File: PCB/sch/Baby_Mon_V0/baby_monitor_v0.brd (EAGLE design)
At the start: 20 x 20 mm, 40 parts, among them J1 BATT-COIN1CR1216, U1 NRF5340-QKAA-AB0-R, U2 MAX30101EFD+, U3 MAX30205MTA+, X1 XRCGB32M000F2P10R0

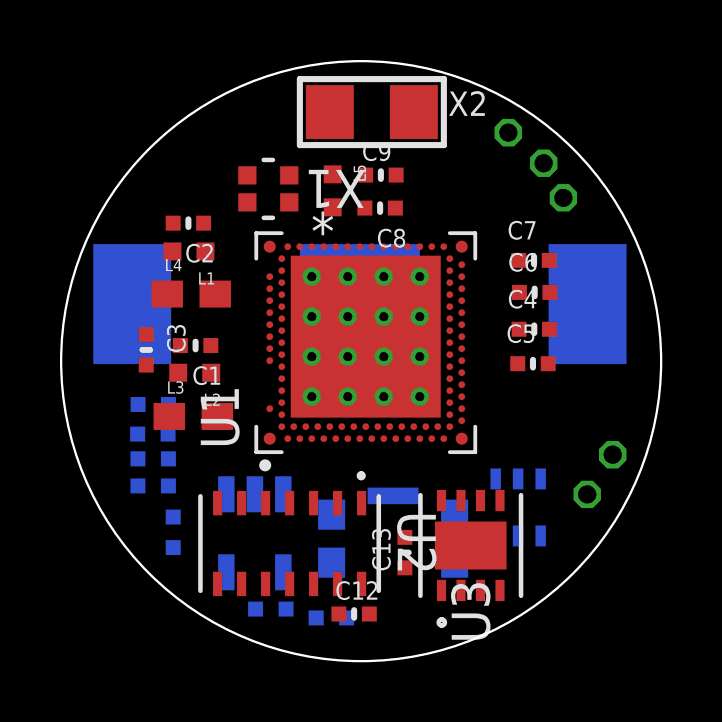
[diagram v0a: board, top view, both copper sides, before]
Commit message: u
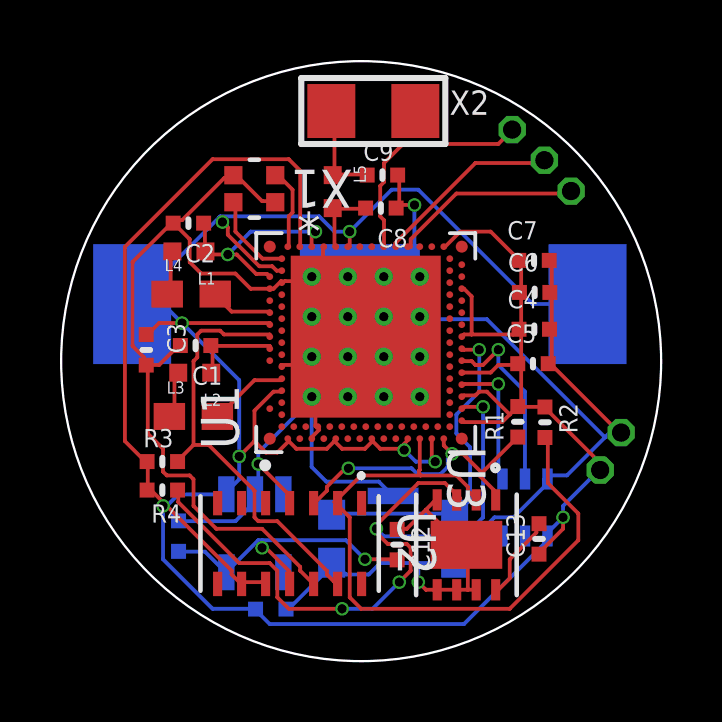
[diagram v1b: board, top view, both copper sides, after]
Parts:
- removed R5: 4.7K, Adafruit Circuit Playground Bluefruit:MICROBUILDER__0402MP
- moved R2 13.1 mm to (12.0, 7.36), flipped to the top, turned to 270 degrees
- moved R1 12.2 mm to (11.1, 7.38), flipped to the top, turned to 90 degrees
- moved C13 4.49 mm to (11.8, 3.47)
- moved C12 2.72 mm to (7.04, 3.28), turned to 270 degrees
- moved J8 0.92 mm to (13.8, 5.77)
- moved J7 0.79 mm to (14.5, 7.02)
- moved X1 0.47 mm to (2.28, 15.1)
- moved J9 0.34 mm to (12.8, 15.1)
- moved R4 0.33 mm to (-0.78, 5.10), flipped to the top, turned to 180 degrees
- moved R3 0.32 mm to (-0.78, 6.05), flipped to the top, turned to 0 degrees
- moved U$2 0.23 mm to (11.3, 4.52)
- moved C11 0.22 mm to (-0.24, 3.56)
- moved J10 0.16 mm to (10.9, 17.1)
- moved U3 0.15 mm to (9.35, 3.27), turned to 270 degrees
- moved J11 0.10 mm to (12.0, 16.1)
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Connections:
- net 3.3V: no longer S1.1, S1.4
- net GND: now also S1.2, S1.3; no longer R5.1
- net SW: now also S1.1, S1.4; no longer R5.2, S1.2, S1.3
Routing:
- net GND: track 0.00 -> 119.6 mm, vias 0 -> 3
- net 3.3V: track 0.00 -> 116.3 mm, vias 0 -> 8
- net OS: track 0.00 -> 25.2 mm, vias 0 -> 4
- net SCL: track 0.00 -> 22.8 mm
- net INT: track 0.00 -> 14.4 mm
- net SW: track 0.00 -> 10.9 mm, vias 0 -> 1
- net SDA: track 0.00 -> 10.4 mm, vias 0 -> 2
- net 1.8V: track 0.00 -> 10.2 mm, vias 0 -> 2
- net N$2: track 0.00 -> 7.65 mm
- net N$8: track 0.00 -> 7.27 mm, vias 0 -> 2
- net N$3: track 0.00 -> 6.40 mm
- net N$1: track 0.00 -> 6.29 mm
- net CI: track 0.00 -> 6.16 mm, vias 0 -> 1
- net DI: track 0.00 -> 4.44 mm, vias 0 -> 1
- net N$13: track 0.00 -> 3.32 mm
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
